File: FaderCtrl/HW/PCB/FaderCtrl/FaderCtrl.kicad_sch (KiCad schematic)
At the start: 52 parts, among them J1 Barrel_Jack_MountingPin, P1 USB_C_Plug_USB2.0, U1 ATxmega256A3BU-A, U4 TSR_1-2450, Y1 32k

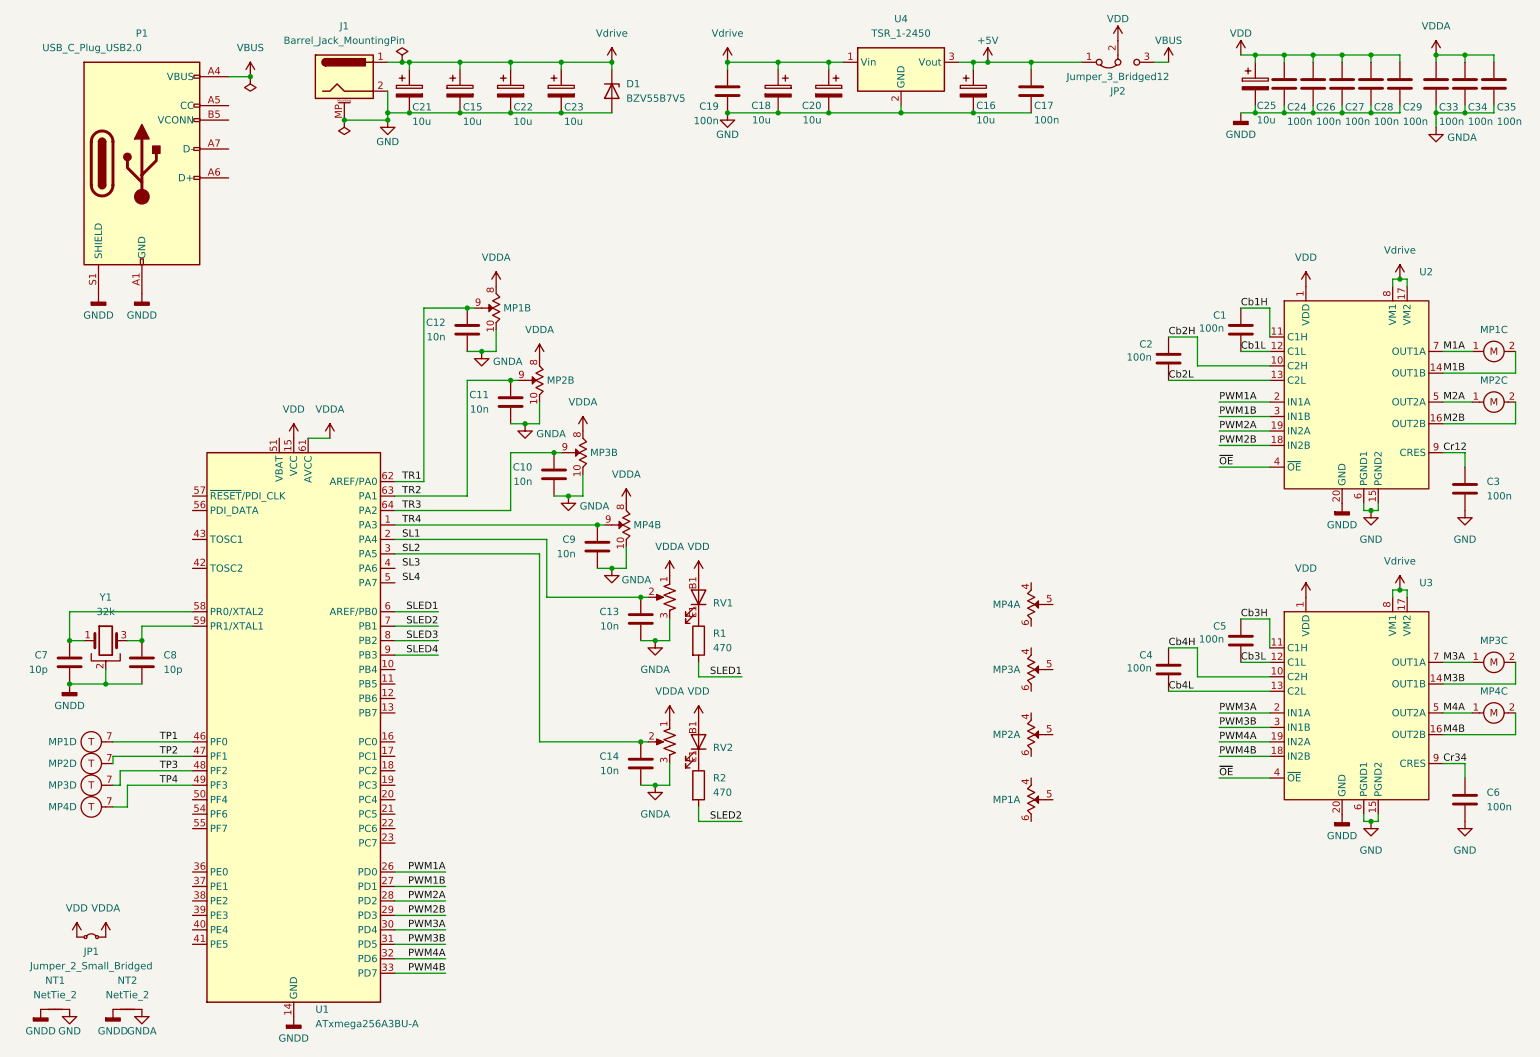
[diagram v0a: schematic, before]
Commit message: a
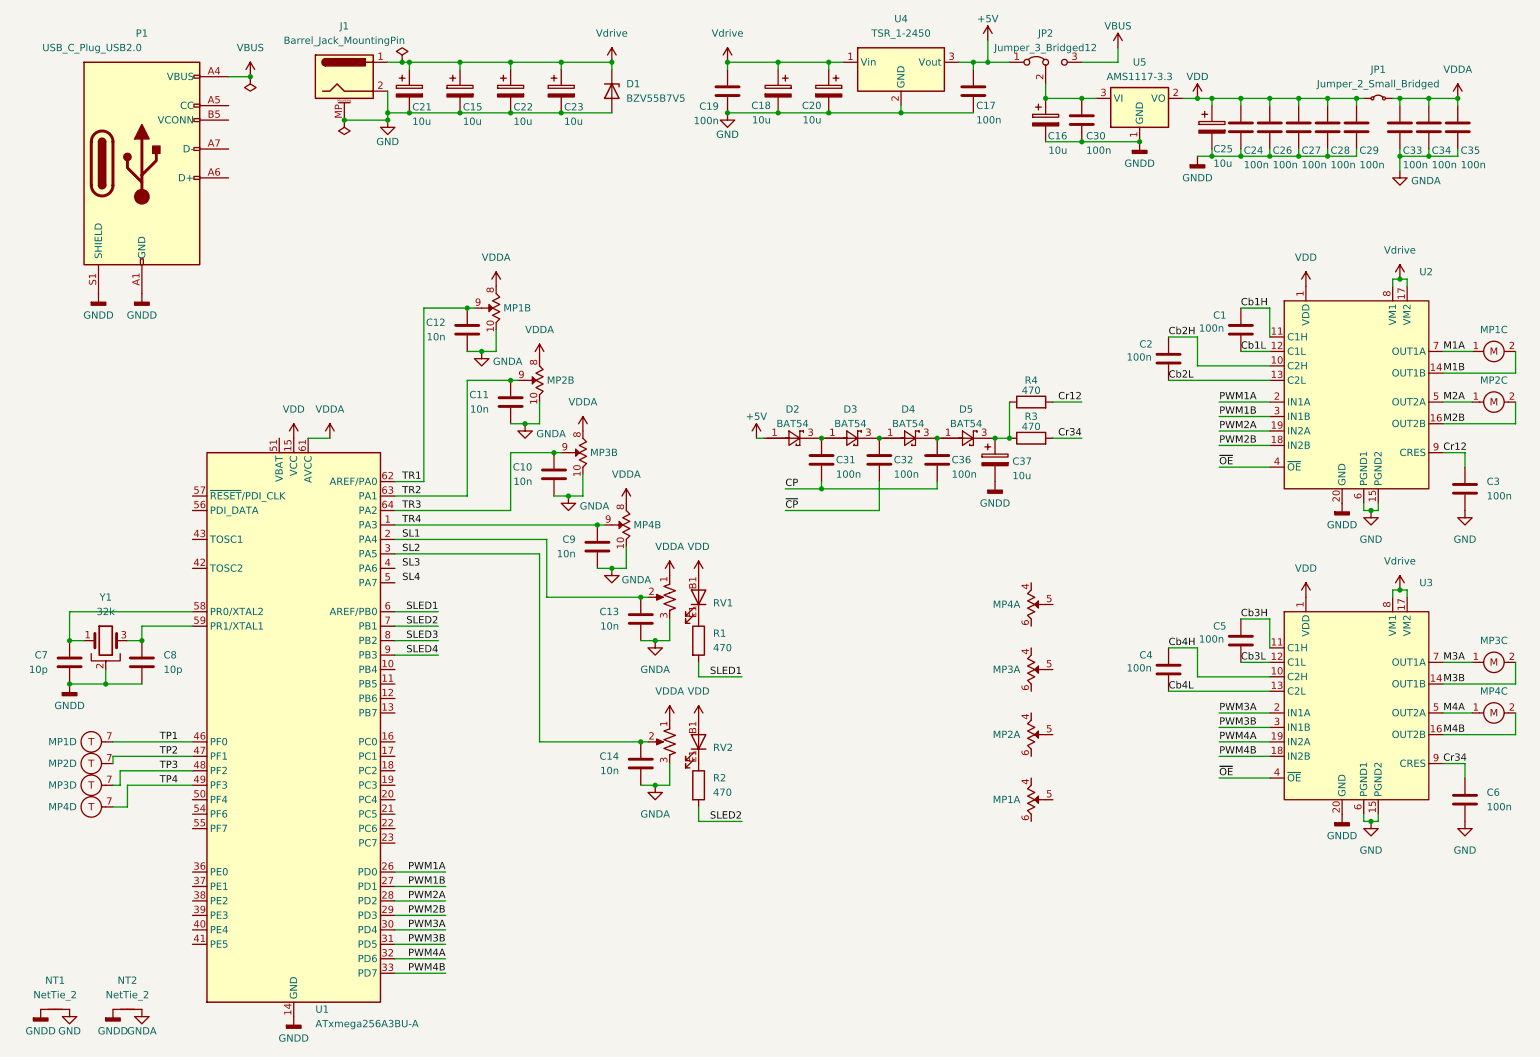
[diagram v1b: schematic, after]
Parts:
- added C30, C31, C32, C36: 100n, Capacitor_SMD:C_0603_1608Metric_Pad1.08x0.95mm_HandSolder, symbol Device:C
- added C37: 10u, Capacitor_SMD:C_0805_2012Metric_Pad1.18x1.45mm_HandSolder, symbol Device:C_Polarized
- added D2, D3, D4, D5: BAT54, Package_TO_SOT_SMD:SOT-323_SC-70, symbol _MYLIBRARY:BAT54
- added R3, R4: 470, Resistor_SMD:R_0603_1608Metric_Pad0.98x0.95mm_HandSolder, symbol Device:R
- added U5: AMS1117-3.3, Package_TO_SOT_SMD:SOT-223-3_TabPin2, symbol Regulator_Linear:AMS1117-3.3
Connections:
- net +5V: now also D2.1; no longer C16.1
- net Cr12: now also R4.2
- net Cr34: now also R3.2
- net GND: no longer C16.2
- net GNDD: now also C16.2, C30.2, C37.2, U5.1 (GND)
- net VDD: now also U5.2 (VO); no longer JP2.2 (C)
- new net: C16.1, C30.1, JP2.2 (C), U5.3 (VI)
- new net: C36.1, D4.3, D5.1
- new net: C37.1, D5.3, R3.1, R4.1
- new net: C31.1, D2.3, D3.1
- new net: C32.1, D3.3, D4.1
- new net CP: C31.2, C36.2
- new net ~{CP}: C32.2
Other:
- moved on the sheet: C16, C17, C24, C25, C26, C27, C28, C29, C33, C34, C35, JP1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
